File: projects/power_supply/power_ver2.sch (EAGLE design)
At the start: 29 parts

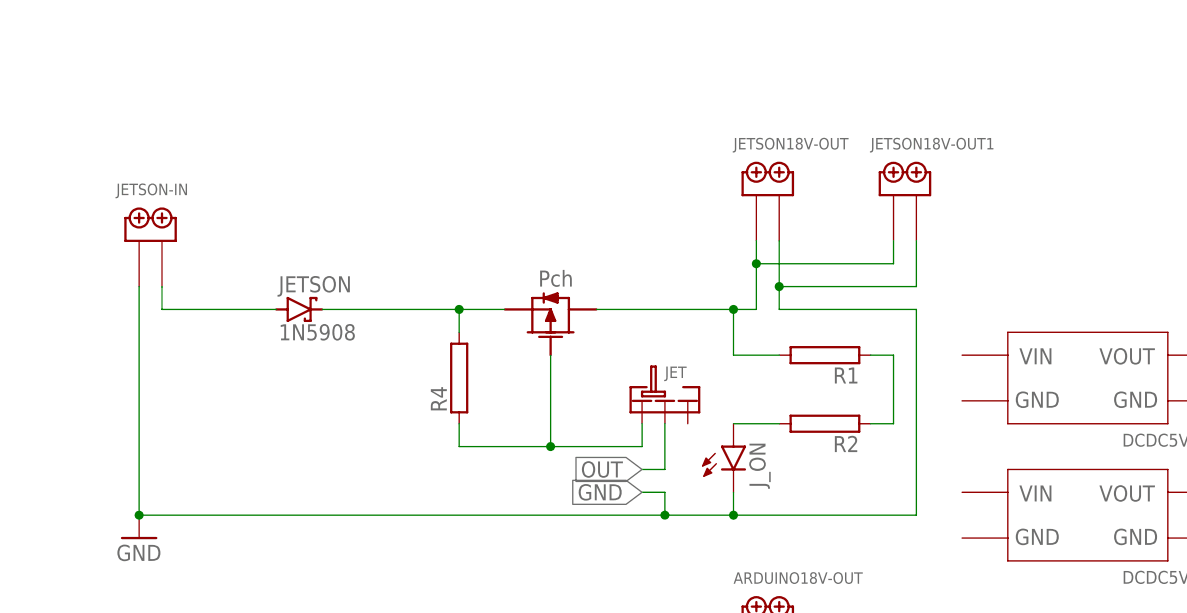
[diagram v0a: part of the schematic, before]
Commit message: aa
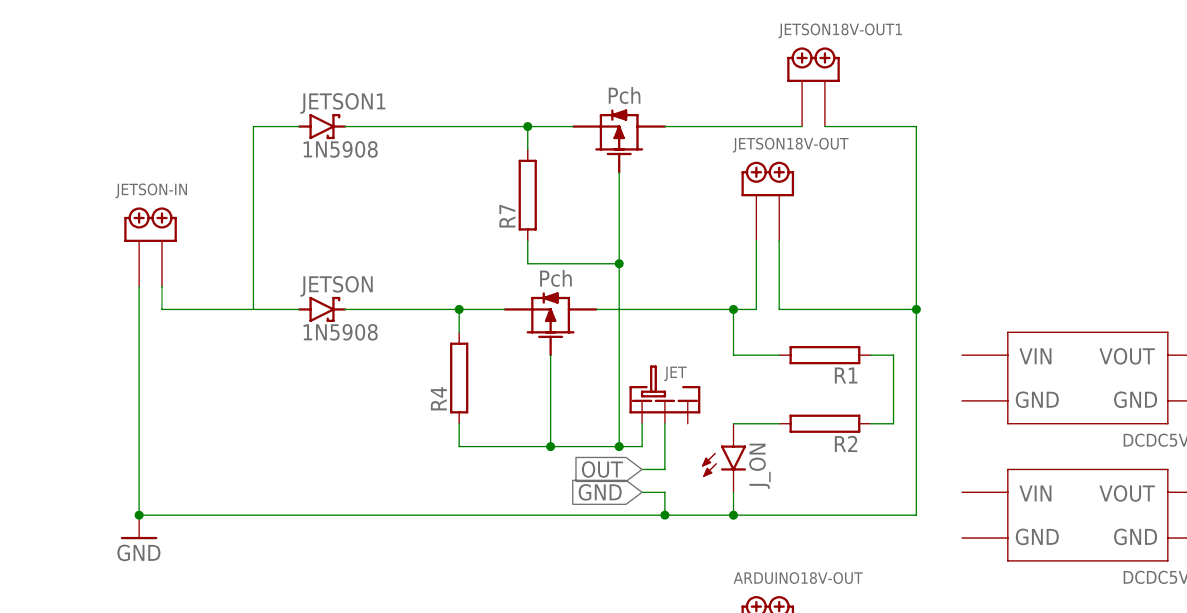
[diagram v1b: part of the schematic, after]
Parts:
- added JETSON1: 1N5908, diode:1N5908
- added R7: (no value), resistor-power:RAC01
- added U$1: 2SJ334, 2SJ334:2SJ334
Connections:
- removed net N$43: JET.L, R4.1, U$4.GATE
- new net MA1: JETSON1.C, R7.2, U$1.SOURCE
- new net N$4: JET.L, R4.1, R7.1, U$1.GATE, U$4.GATE
- new net N$5: JETSON18V-OUT1.P$1, U$1.DRAIN
- net 18V: now also JETSON1.A
- net MAC: no longer JETSON18V-OUT1.P$1
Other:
- moved on the sheet: JETSON, JETSON18V-OUT1
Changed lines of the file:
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@@
 <part name="GND10" library="supply1" library_urn="urn:adsk.eagle:library:371" deviceset="GND" device=""/>
 <part name="JETSON18V-OUT1" library="TB113-2B-x-x-0-x-x" library_urn="urn:adsk.eagle:library:38507486" deviceset="2PIN" device="" package3d_urn="urn:adsk.eagle:package:38507490/6" override_package3d_urn="urn:adsk.eagle:package:38731294/2" override_package_urn="urn:adsk.eagle:footprint:38731295/1"/>
+<part name="U$1" library="2SJ334" deviceset="2SJ334" device="" package3d_urn="urn:adsk.eagle:package:38731260/2"/>
+<part name="R7" library="resistor-power" library_urn="urn:adsk.eagle:library:344" deviceset="R" device="AC01" package3d_urn="urn:adsk.eagle:package:25124/1"/>
+<part name="JETSON1" library="diode" library_urn="urn:adsk.eagle:library:210" deviceset="1N5908" device="" package3d_urn="urn:adsk.eagle:package:43355/2"/>
 </parts>
 <sheets>
@@
 </instance>
 <instance part="GND2" gate="1" x="45.72" y="-7.62" smashed="yes"/>
-<instance part="JETSON" gate="1" x="63.5" y="68.58" smashed="yes">
-<attribute name="NAME" x="61.214" y="70.485" size="1.778" layer="95"/>
-<attribute name="VALUE" x="61.214" y="65.151" size="1.778" layer="96"/>
+<instance part="JETSON" gate="1" x="66.04" y="68.58" smashed="yes">
+<attribute name="NAME" x="63.754" y="70.485" size="1.778" layer="95"/>
+<attribute name="VALUE" x="63.754" y="65.151" size="1.778" layer="96"/>
 </instance>
 <instance part="ARDUINO" gate="1" x="63.5" y="17.78" smashed="yes">
@@
 <attribute name="VALUE" x="215.9" y="2.54" size="1.778" layer="96"/>
 </instance>
-<instance part="JETSON18V-OUT1" gate="G$1" x="129.54" y="81.28" smashed="yes">
-<attribute name="NAME" x="127" y="86.36" size="1.27" layer="95"/>
+<instance part="JETSON18V-OUT1" gate="G$1" x="119.38" y="93.98" smashed="yes">
+<attribute name="NAME" x="116.84" y="99.06" size="1.27" layer="95"/>
+</instance>
+<instance part="U$1" gate="G$1" x="104.14" y="83.82" smashed="yes" rot="MR0"/>
+<instance part="R7" gate="G$1" x="88.9" y="81.28" smashed="yes" rot="R90">
+<attribute name="NAME" x="87.5284" y="77.47" size="1.778" layer="95" rot="R90"/>
+<attribute name="VALUE" x="91.821" y="77.47" size="1.778" layer="96" rot="R90"/>
+</instance>
+<instance part="JETSON1" gate="1" x="66.04" y="88.9" smashed="yes">
+<attribute name="NAME" x="63.754" y="90.805" size="1.778" layer="95"/>
+<attribute name="VALUE" x="63.754" y="85.471" size="1.778" layer="96"/>
 </instance>
 </instances>
@@
 </busses>
 <nets>
-<net name="N$43" class="1">
-<segment>
-<pinref part="U$4" gate="G$1" pin="GATE"/>
-<wire x1="91.44" y1="63.5" x2="91.44" y2="53.34" width="0.1524" layer="91"/>
-<pinref part="JET" gate="G$1" pin="L"/>
-<wire x1="91.44" y1="53.34" x2="101.6" y2="53.34" width="0.1524" layer="91"/>
-<wire x1="101.6" y1="53.34" x2="101.6" y2="55.88" width="0.1524" layer="91"/>
-<wire x1="81.28" y1="55.88" x2="81.28" y2="53.34" width="0.1524" layer="91"/>
-<wire x1="81.28" y1="53.34" x2="91.44" y2="53.34" width="0.1524" layer="91"/>
-<junction x="91.44" y="53.34"/>
-<pinref part="R4" gate="G$1" pin="1"/>
-</segment>
-</net>
 <net name="MA" class="1">
 <segment>
@@
 <pinref part="R4" gate="G$1" pin="2"/>
 <pinref part="JETSON" gate="1" pin="C"/>
-<wire x1="66.04" y1="68.58" x2="81.28" y2="68.58" width="0.1524" layer="91"/>
+<wire x1="68.58" y1="68.58" x2="81.28" y2="68.58" width="0.1524" layer="91"/>
 </segment>
 </net>
@@
 <pinref part="JETSON-IN" gate="G$1" pin="P$2"/>
 <pinref part="JETSON" gate="1" pin="A"/>
-<wire x1="48.26" y1="68.58" x2="60.96" y2="68.58" width="0.1524" layer="91"/>
+<wire x1="58.42" y1="68.58" x2="63.5" y2="68.58" width="0.1524" layer="91"/>
+<wire x1="48.26" y1="68.58" x2="58.42" y2="68.58" width="0.1524" layer="91"/>
+<wire x1="58.42" y1="68.58" x2="58.42" y2="88.9" width="0.1524" layer="91"/>
+<pinref part="JETSON1" gate="1" pin="A"/>
+<wire x1="58.42" y1="88.9" x2="63.5" y2="88.9" width="0.1524" layer="91"/>
 </segment>
 </net>
 <net name="MAC" class="1">
 <segment>
-<pinref part="U$4" gate="G$1" pin="DRAIN"/>
-<wire x1="96.52" y1="68.58" x2="111.76" y2="68.58" width="0.1524" layer="91"/>
 <wire x1="111.76" y1="68.58" x2="114.3" y2="68.58" width="0.1524" layer="91"/>
-<wire x1="114.3" y1="68.58" x2="114.3" y2="73.66" width="0.1524" layer="91"/>
-<wire x1="114.3" y1="73.66" x2="114.3" y2="76.2" width="0.1524" layer="91"/>
-<junction x="111.76" y="68.58"/>
+<wire x1="114.3" y1="68.58" x2="114.3" y2="76.2" width="0.1524" layer="91"/>
 <pinref part="JETSON18V-OUT" gate="G$1" pin="P$1"/>
 <wire x1="111.76" y1="68.58" x2="111.76" y2="63.5" width="0.1524" layer="91"/>
 <wire x1="111.76" y1="63.5" x2="116.84" y2="63.5" width="0.1524" layer="91"/>
 <pinref part="R1" gate="G$1" pin="2"/>
-<wire x1="114.3" y1="73.66" x2="129.54" y2="73.66" width="0.1524" layer="91"/>
-<junction x="114.3" y="73.66"/>
-<pinref part="JETSON18V-OUT1" gate="G$1" pin="P$1"/>
-<wire x1="129.54" y1="73.66" x2="129.54" y2="76.2" width="0.1524" layer="91"/>
+<pinref part="U$4" gate="G$1" pin="DRAIN"/>
+<wire x1="96.52" y1="68.58" x2="111.76" y2="68.58" width="0.1524" layer="91"/>
+<junction x="111.76" y="68.58"/>
 </segment>
 </net>
@@
 <segment>
 <wire x1="104.14" y1="45.72" x2="45.72" y2="45.72" width="0.1524" layer="91"/>
-<wire x1="116.84" y1="76.2" x2="116.84" y2="71.12" width="0.1524" layer="91"/>
-<wire x1="116.84" y1="71.12" x2="116.84" y2="68.58" width="0.1524" layer="91"/>
+<wire x1="116.84" y1="76.2" x2="116.84" y2="68.58" width="0.1524" layer="91"/>
 <wire x1="116.84" y1="68.58" x2="132.08" y2="68.58" width="0.1524" layer="91"/>
 <wire x1="132.08" y1="68.58" x2="132.08" y2="45.72" width="0.1524" layer="91"/>
@@
 <pinref part="GND1" gate="1" pin="GND"/>
 <junction x="45.72" y="45.72"/>
-<wire x1="116.84" y1="71.12" x2="132.08" y2="71.12" width="0.1524" layer="91"/>
-<junction x="116.84" y="71.12"/>
 <pinref part="JETSON18V-OUT1" gate="G$1" pin="P$2"/>
-<wire x1="132.08" y1="71.12" x2="132.08" y2="76.2" width="0.1524" layer="91"/>
+<wire x1="121.92" y1="88.9" x2="132.08" y2="88.9" width="0.1524" layer="91"/>
+<wire x1="132.08" y1="88.9" x2="132.08" y2="68.58" width="0.1524" layer="91"/>
+<junction x="132.08" y="68.58"/>
 </segment>
 <segment>
@@
 </segment>
 </net>
+<net name="N$4" class="1">
+<segment>
+<pinref part="U$1" gate="G$1" pin="GATE"/>
+<wire x1="99.06" y1="83.82" x2="99.06" y2="73.66" width="0.1524" layer="91"/>
+<wire x1="88.9" y1="76.2" x2="88.9" y2="73.66" width="0.1524" layer="91"/>
+<wire x1="88.9" y1="73.66" x2="99.06" y2="73.66" width="0.1524" layer="91"/>
+<pinref part="R7" gate="G$1" pin="1"/>
+<pinref part="U$4" gate="G$1" pin="GATE"/>
+<pinref part="JET" gate="G$1" pin="L"/>
+<wire x1="91.44" y1="63.5" x2="91.44" y2="53.34" width="0.1524" layer="91"/>
+<wire x1="91.44" y1="53.34" x2="99.06" y2="53.34" width="0.1524" layer="91"/>
+<wire x1="99.06" y1="53.34" x2="101.6" y2="53.34" width="0.1524" layer="91"/>
+<wire x1="101.6" y1="53.34" x2="101.6" y2="55.88" width="0.1524" layer="91"/>
+<wire x1="81.28" y1="55.88" x2="81.28" y2="53.34" width="0.1524" layer="91"/>
+<wire x1="81.28" y1="53.34" x2="91.44" y2="53.34" width="0.1524" layer="91"/>
+<junction x="91.44" y="53.34"/>
+<pinref part="R4" gate="G$1" pin="1"/>
+<wire x1="99.06" y1="73.66" x2="99.06" y2="53.34" width="0.1524" layer="91"/>
+<junction x="99.06" y="73.66"/>
+<junction x="99.06" y="53.34"/>
+</segment>
+</net>
+<net name="MA1" class="1">
+<segment>
+<pinref part="U$1" gate="G$1" pin="SOURCE"/>
+<wire x1="88.9" y1="88.9" x2="93.98" y2="88.9" width="0.1524" layer="91"/>
+<wire x1="88.9" y1="86.36" x2="88.9" y2="88.9" width="0.1524" layer="91"/>
+<junction x="88.9" y="88.9"/>
+<pinref part="R7" gate="G$1" pin="2"/>
+<pinref part="JETSON1" gate="1" pin="C"/>
+<wire x1="68.58" y1="88.9" x2="88.9" y2="88.9" width="0.1524" layer="91"/>
+</segment>
+</net>
+<net name="N$5" class="0">
+<segment>
+<pinref part="U$1" gate="G$1" pin="DRAIN"/>
+<pinref part="JETSON18V-OUT1" gate="G$1" pin="P$1"/>
+<wire x1="104.14" y1="88.9" x2="119.38" y2="88.9" width="0.1524" layer="91"/>
+</segment>
+</net>
